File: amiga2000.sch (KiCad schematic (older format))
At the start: 0 parts

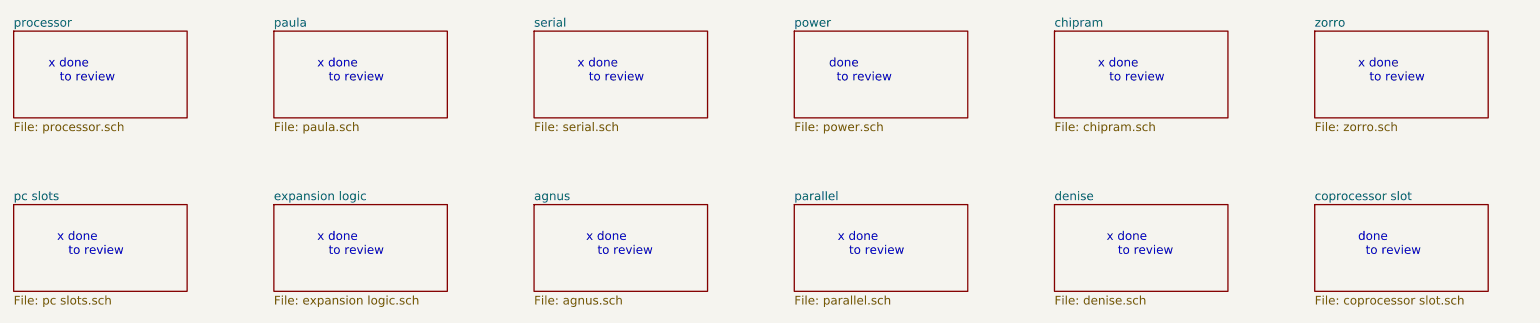
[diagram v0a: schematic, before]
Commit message: urgh
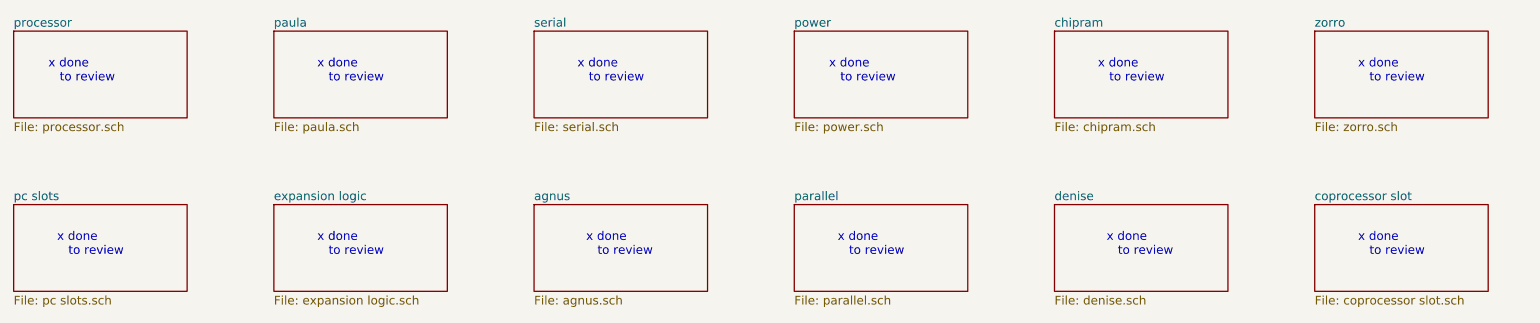
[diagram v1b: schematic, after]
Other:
- note removed: "done\n to review"
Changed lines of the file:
@@
 x done\n   to review
 Text Notes 5700 1300 0    50   ~ 0
-  done\n  to review
+x done\n   to review
 Text Notes 7250 1300 0    50   ~ 0
 x done\n   to review
@@
 x done\n   to review
 Text Notes 8750 2300 0    50   ~ 0
-  done\n  to review
+ x done\n   to review
 Text Notes 7300 2300 0    50   ~ 0
 x done\n   to review
